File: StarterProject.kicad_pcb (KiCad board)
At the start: 2 copper layers, 95 x 75 mm, 54 parts, among them J1 POWER_MINION, J10 EX_HDLT, J11 EX_BRAKELIGHT, J12 +12V, J13 GND, J14 POWER_LEADERBOARD, J15 F/R, J16 TURN_SIGNAL, J17 NEU_INDICATOR, J18 FOR_INDICATOR, J19 REV_INDICATOR, J2 CRUISE_SET, J20 CRUZ_SET, J21 CRUZ_EN, J22 REGEN, J3 CRUISE_ENABLE, J4 REGEN, J5 HZD, J6 EX_RIGHTBLINK, J7 EX_LEFTBLINK, J8 IN_RIGHTBLINK, J9 IN_LEFTBLINK, SW1 CRUISE_SET_SW, SW2 CRUISE_ENABLE_SW, SW3 REGEN_SW, SW4 HZD_SW, SW5 F/R, SW6 TURN_SIGNAL_SW

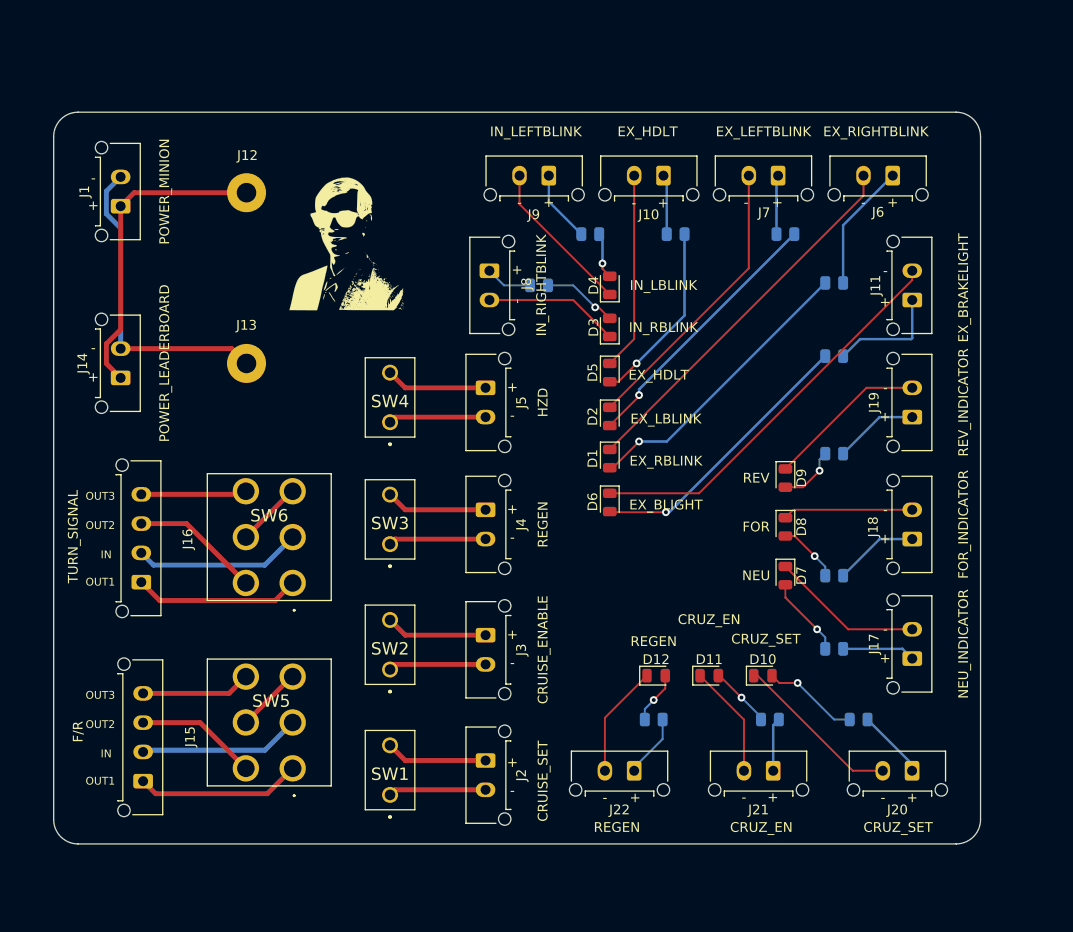
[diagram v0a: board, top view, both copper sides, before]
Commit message: Updated PCB
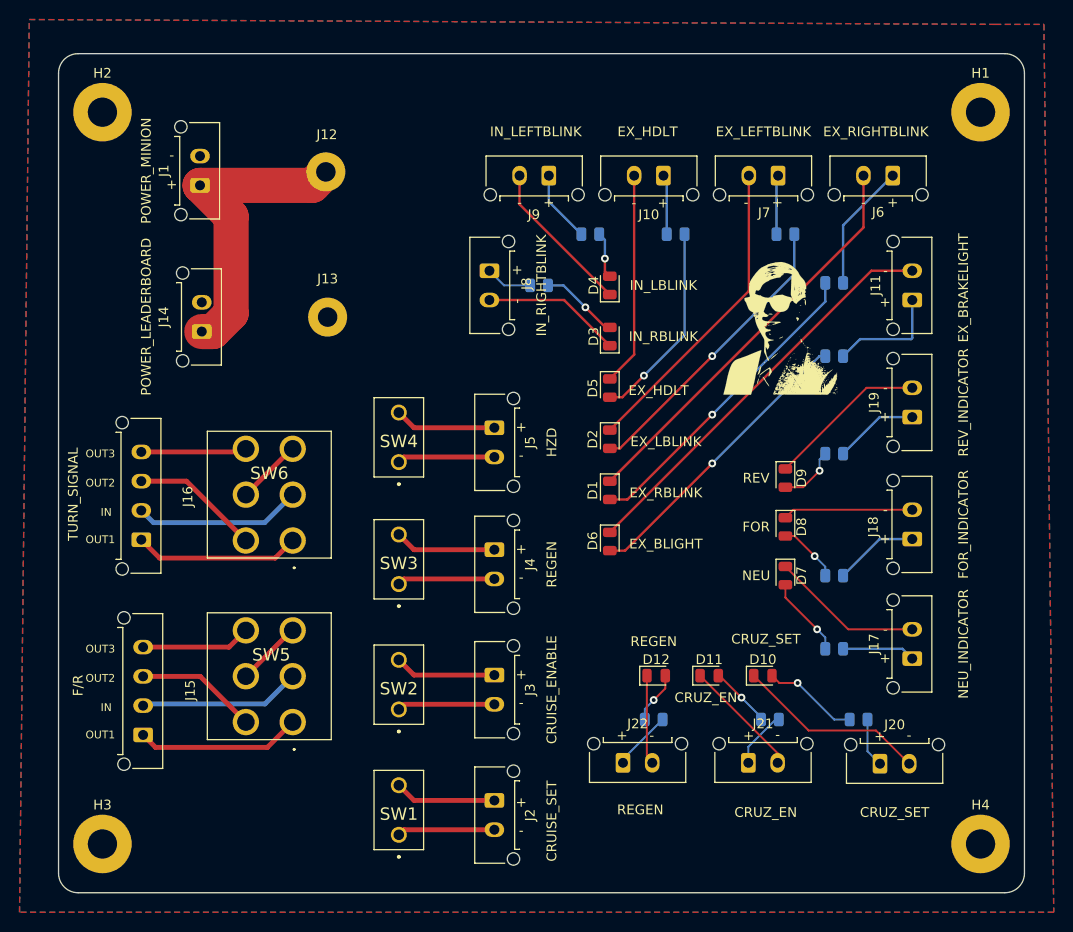
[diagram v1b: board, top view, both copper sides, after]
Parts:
- added H1: MountingHole, MountingHole:MountingHole_3mm_Pad, F.Cu at (125.0, 32.5)
- added H2: MountingHole, MountingHole:MountingHole_3mm_Pad, F.Cu at (35.0, 32.5)
- added H3: MountingHole, MountingHole:MountingHole_3mm_Pad, F.Cu at (35.0, 107.5)
- added H4: MountingHole, MountingHole:MountingHole_3mm_Pad, F.Cu at (125.0, 107.5)
- moved LOGO1 45.3 mm to (104.0, 54.5)
- moved J13 9.57 mm to (58.1, 53.5)
- moved J14 9.57 mm to (45.2, 55.0)
- moved J1 8.41 mm to (45.0, 40.0)
- moved J12 8.41 mm to (57.9, 38.6)
- moved J15 4.74 mm to (39.2, 96.3)
- moved SW5 4.74 mm to (54.5, 95.0)
- moved J16 4.35 mm to (39.0, 76.3)
- moved SW6 4.35 mm to (54.5, 76.4)
- moved J2 4.19 mm to (75.2, 103.0)
- moved J3 4.19 mm to (75.2, 90.2)
- moved J4 4.19 mm to (75.2, 77.3)
- moved J5 4.19 mm to (75.2, 64.8)
- moved SW1 4.19 mm to (65.4, 106.6)
- moved SW2 4.19 mm to (65.4, 93.7)
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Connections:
- net Net-(J1-Pad2) renamed GND
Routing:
- net GND: track 32.3 -> 0.00 mm
- net Net-(D1-Pad1): track 38.9 -> 42.1 mm
- net Net-(D2-Pad2): track 27.5 -> 30.4 mm
- net Net-(D1-Pad2): track 29.9 -> 32.4 mm
- net Net-(D10-Pad1): track 17.3 -> 19.7 mm
- net Net-(D2-Pad1): track 29.7 -> 32.0 mm
- net Net-(J20-Pad1): track 7.14 -> 5.06 mm
- net Net-(D12-Pad1): track 11.2 -> 9.15 mm
- net Net-(D5-Pad2): track 18.8 -> 20.6 mm
- net Net-(D6-Pad2): track 28.7 -> 30.3 mm
- net Net-(D5-Pad1): track 20.3 -> 21.9 mm
- net Net-(D6-Pad1): track 41.0 -> 42.1 mm
- net Net-(D11-Pad1): track 11.5 -> 12.2 mm
- net Net-(J1-Pad1): track 32.3 -> 31.7 mm
- added copper zone on B.Cu, net GND
- added copper zone on F.Cu, net GND
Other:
- board size 95 x 75 mm -> 99 x 86 mm
- board text added: "UTSVT- Controls Minion Test v0.1 Pratyush Patra"
